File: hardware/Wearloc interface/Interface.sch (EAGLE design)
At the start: 21 parts, among them U1 PCA9306DCT, U2 LTC2804-1GN, U3 TXB0104D

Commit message: interface board work in progress
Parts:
- added C10, C9: (no value), rcl:C-EUC0805K
- added R10, R8, R9: (no value), rcl:R-EU_R0805
- added U4: MCP1826ADJ, wearloc:MCP1826ADJ
- added USB2: MOLEX-47346-0001, wearloc:MOLEX-47346-0001
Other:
- note added: "Jennifer Nist Universität Freiburg"
- note added: "Logic converters"
- note added: "Power supply and connectors"
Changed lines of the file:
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@@
 <part name="R6" library="rcl" deviceset="R-EU_" device="R0805"/>
 <part name="R7" library="rcl" deviceset="R-EU_" device="R0805"/>
+<part name="FRAME1" library="frames" deviceset="A4L-LOC" device=""/>
+<part name="FRAME2" library="frames" deviceset="A4L-LOC" device=""/>
+<part name="USB2" library="wearloc" deviceset="MOLEX-47346-0001" device=""/>
+<part name="U4" library="wearloc" deviceset="MCP1826" device="ADJ"/>
 <part name="JP1" library="wearloc" deviceset="INTEL_EDISON_BB_HEADER" device=""/>
-<part name="FRAME1" library="frames" deviceset="A4L-LOC" device=""/>
 <part name="USB1" library="wearloc" deviceset="MOLEX-47346-0001" device=""/>
+<part name="R8" library="rcl" deviceset="R-EU_" device="R0805"/>
+<part name="R9" library="rcl" deviceset="R-EU_" device="R0805"/>
+<part name="R10" library="rcl" deviceset="R-EU_" device="R0805"/>
+<part name="C9" library="rcl" deviceset="C-EU" device="C0805K"/>
+<part name="C10" library="rcl" deviceset="C-EU" device="C0805K"/>
 </parts>
 <sheets>
 <sheet>
 <plain>
+<text x="165.1" y="10.16" size="3.81" layer="94">Jennifer Nist
+Universität Freiburg</text>
+<text x="217.17" y="20.32" size="2.1844" layer="94">Logic converters</text>
 </plain>
 <instances>
-<instance part="U1" gate="PCA9306" x="50.8" y="160.02"/>
-<instance part="U2" gate="LTC2804-1" x="33.02" y="45.72"/>
-<instance part="U3" gate="TXB0104" x="25.4" y="121.92"/>
-<instance part="C1" gate="G$1" x="68.58" y="139.7"/>
-<instance part="R1" gate="G$1" x="83.82" y="96.52"/>
-<instance part="L1" gate="LQH2MC" x="71.12" y="60.96" rot="R90"/>
-<instance part="C2" gate="G$1" x="68.58" y="129.54"/>
-<instance part="C3" gate="G$1" x="68.58" y="119.38"/>
-<instance part="C4" gate="G$1" x="68.58" y="109.22"/>
-<instance part="C5" gate="G$1" x="55.88" y="109.22"/>
-<instance part="C6" gate="G$1" x="55.88" y="119.38"/>
-<instance part="C7" gate="G$1" x="55.88" y="129.54"/>
-<instance part="C8" gate="G$1" x="55.88" y="139.7"/>
-<instance part="R2" gate="G$1" x="83.82" y="88.9"/>
-<instance part="R3" gate="G$1" x="83.82" y="81.28"/>
-<instance part="R4" gate="G$1" x="83.82" y="73.66"/>
-<instance part="R5" gate="G$1" x="71.12" y="73.66"/>
-<instance part="R6" gate="G$1" x="71.12" y="81.28"/>
-<instance part="R7" gate="G$1" x="71.12" y="88.9"/>
-<instance part="JP1" gate="J17" x="111.76" y="45.72"/>
-<instance part="JP1" gate="J18" x="142.24" y="45.72"/>
-<instance part="JP1" gate="J19" x="177.8" y="45.72"/>
-<instance part="JP1" gate="J20" x="215.9" y="45.72"/>
+<instance part="U1" gate="PCA9306" x="203.2" y="134.62"/>
+<instance part="U2" gate="LTC2804-1" x="33.02" y="114.3"/>
+<instance part="U3" gate="TXB0104" x="142.24" y="68.58"/>
+<instance part="C1" gate="G$1" x="25.4" y="165.1"/>
+<instance part="R1" gate="G$1" x="60.96" y="152.4"/>
+<instance part="L1" gate="LQH2MC" x="38.1" y="152.4" rot="R90"/>
+<instance part="C2" gate="G$1" x="38.1" y="165.1"/>
+<instance part="C3" gate="G$1" x="53.34" y="165.1"/>
+<instance part="C4" gate="G$1" x="68.58" y="165.1"/>
+<instance part="C5" gate="G$1" x="83.82" y="165.1"/>
+<instance part="C6" gate="G$1" x="231.14" y="162.56"/>
+<instance part="C7" gate="G$1" x="170.18" y="83.82"/>
+<instance part="C8" gate="G$1" x="182.88" y="83.82"/>
+<instance part="R2" gate="G$1" x="180.34" y="165.1"/>
+<instance part="R3" gate="G$1" x="180.34" y="157.48"/>
+<instance part="R4" gate="G$1" x="195.58" y="165.1"/>
+<instance part="R5" gate="G$1" x="195.58" y="157.48"/>
+<instance part="R6" gate="G$1" x="213.36" y="165.1"/>
+<instance part="R7" gate="G$1" x="175.26" y="71.12"/>
 <instance part="FRAME1" gate="G$1" x="0" y="0"/>
-<instance part="USB1" gate="MICRO-USB" x="99.06" y="147.32"/>
+</instances>
+<busses>
+</busses>
+<nets>
+</nets>
+</sheet>
+<sheet>
+<plain>
+<text x="165.1" y="10.16" size="3.81" layer="94">Jennifer Nist
+Universität Freiburg</text>
+<text x="215.9" y="20.32" size="2.1844" layer="94">Power supply and connectors</text>
+</plain>
+<instances>
+<instance part="FRAME2" gate="G$1" x="0" y="0"/>
+<instance part="USB2" gate="MICRO-USB" x="-33.02" y="144.78"/>
+<instance part="U4" gate="MCP1826" x="172.72" y="139.7"/>
+<instance part="JP1" gate="J17" x="48.26" y="40.64"/>
+<instance part="JP1" gate="J18" x="78.74" y="40.64"/>
+<instance part="JP1" gate="J19" x="114.3" y="40.64"/>
+<instance part="JP1" gate="J20" x="152.4" y="40.64"/>
+<instance part="USB1" gate="MICRO-USB" x="35.56" y="142.24"/>
+<instance part="R8" gate="G$1" x="203.2" y="152.4"/>
+<instance part="R9" gate="G$1" x="203.2" y="142.24"/>
+<instance part="R10" gate="G$1" x="203.2" y="132.08"/>
+<instance part="C9" gate="G$1" x="137.16" y="149.86"/>
+<instance part="C10" gate="G$1" x="137.16" y="137.16"/>
 </instances>
 <busses>
@@
 </schematic>
 </drawing>
+<compatibility>
+<note version="6.3" minversion="6.2.2" severity="warning">
+Since Version 6.2.2 text objects can contain more than one line,
+which will not be processed correctly with this version.
+</note>
+</compatibility>
 </eagle>

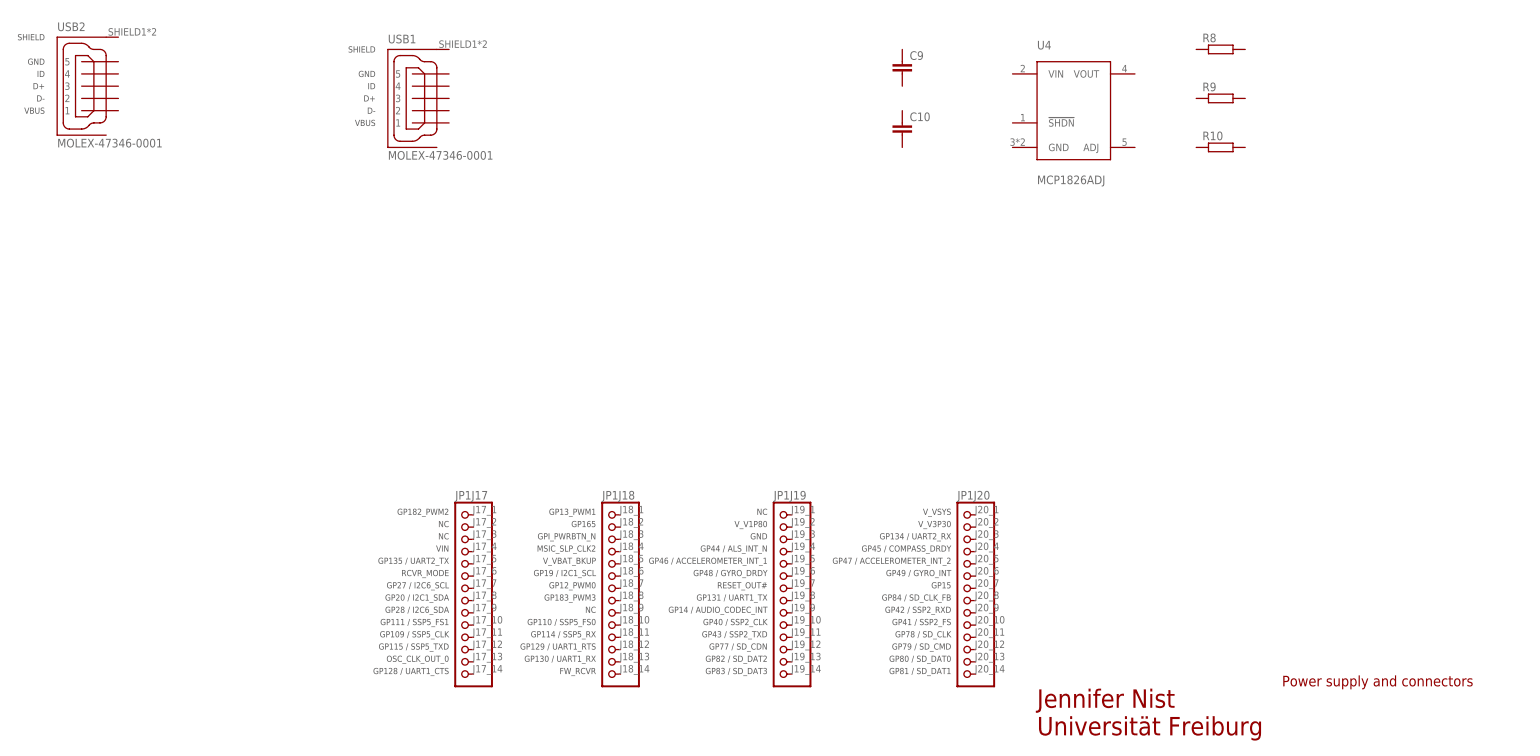
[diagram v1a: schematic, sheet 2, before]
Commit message: worked on schematic
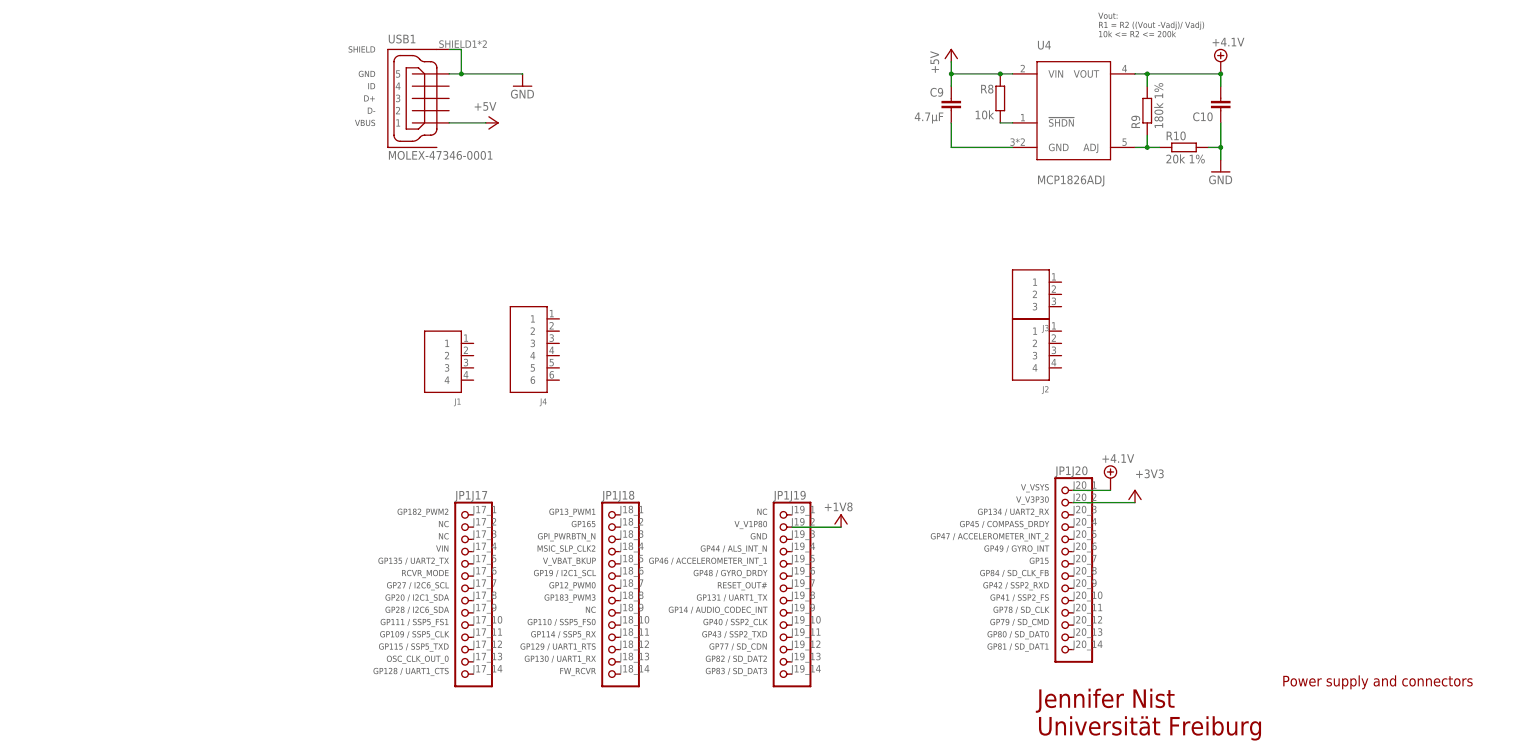
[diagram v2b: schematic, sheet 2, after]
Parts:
- removed USB2: MOLEX-47346-0001, wearloc:MOLEX-47346-0001
- added J1, J2: S4B-XH-A90°, wearloc:S4B-XH-A90°
- added J3: S3B-XH-A90°, wearloc:S3B-XH-A90°
- added J4: S6B-XH-A90°, wearloc:S6B-XH-A90°
- C9: value (none) -> 4.7µF
- R10: value (none) -> 20k 1%
- R8: value (none) -> 10k
- R9: value (none) -> 180k 1%
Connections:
- new net +1V8: JP1J19.2
- new net +3V3: JP1J20.2
- new net +4.1V: C10.2, JP1J20.1, R9.2, U4.VOUT
- new net +5V: C9.1, R8.2, U4.VIN, USB1.1
- new net GND: C10.1, R10.2, USB1.5, USB1.SHIELD
- new net N$1: C9.2, U4.GND
- new net N$2: R8.1, U4.!SHDN
- new net N$4: R10.1, R9.1, U4.ADJ
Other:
- note added: "Vout: R1 = R2 ((Vout -Vadj)/ Vadj) 10k <= R2 <= 200k"
- moved on the sheet: C10, C9, JP1J20, R10, R8, R9
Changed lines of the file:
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@@
 <part name="FRAME1" library="frames" deviceset="A4L-LOC" device=""/>
 <part name="FRAME2" library="frames" deviceset="A4L-LOC" device=""/>
-<part name="USB2" library="wearloc" deviceset="MOLEX-47346-0001" device=""/>
 <part name="U4" library="wearloc" deviceset="MCP1826" device="ADJ"/>
 <part name="JP1" library="wearloc" deviceset="INTEL_EDISON_BB_HEADER" device=""/>
 <part name="USB1" library="wearloc" deviceset="MOLEX-47346-0001" device=""/>
-<part name="R8" library="rcl" deviceset="R-EU_" device="R0805"/>
-<part name="R9" library="rcl" deviceset="R-EU_" device="R0805"/>
-<part name="R10" library="rcl" deviceset="R-EU_" device="R0805"/>
-<part name="C9" library="rcl" deviceset="C-EU" device="C0805K"/>
+<part name="R8" library="rcl" deviceset="R-EU_" device="R0805" value="10k"/>
+<part name="R9" library="rcl" deviceset="R-EU_" device="R0805" value="180k 1%"/>
+<part name="R10" library="rcl" deviceset="R-EU_" device="R0805" value="20k 1%"/>
+<part name="C9" library="rcl" deviceset="C-EU" device="C0805K" value="4.7µF"/>
 <part name="C10" library="rcl" deviceset="C-EU" device="C0805K"/>
+<part name="J1" library="wearloc" deviceset="S4B-XH-A" device="90°"/>
+<part name="J2" library="wearloc" deviceset="S4B-XH-A" device="90°"/>
+<part name="J3" library="wearloc" deviceset="S3B-XH-A" device="90°"/>
+<part name="J4" library="wearloc" deviceset="S6B-XH-A" device="90°"/>
+<part name="P+1" library="supply1" deviceset="+5V" device=""/>
+<part name="GND1" library="supply1" deviceset="GND" device=""/>
+<part name="P+2" library="supply1" deviceset="+5V" device=""/>
+<part name="GND2" library="supply1" deviceset="GND" device=""/>
+<part name="SUPPLY1" library="supply2" deviceset="+4.1V" device=""/>
+<part name="SUPPLY2" library="supply2" deviceset="+4.1V" device=""/>
+<part name="+3V1" library="supply1" deviceset="+3V3" device=""/>
+<part name="+1V1" library="wearloc" deviceset="+1V8" device=""/>
 </parts>
 <sheets>
@@
 Universität Freiburg</text>
 <text x="215.9" y="20.32" size="2.1844" layer="94">Power supply and connectors</text>
+<text x="177.8" y="154.94" size="1.27" layer="97">Vout:
+R1 = R2 ((Vout -Vadj)/ Vadj)
+10k &lt;= R2 &lt;= 200k</text>
 </plain>
 <instances>
 <instance part="FRAME2" gate="G$1" x="0" y="0"/>
-<instance part="USB2" gate="MICRO-USB" x="-33.02" y="144.78"/>
 <instance part="U4" gate="MCP1826" x="172.72" y="139.7"/>
 <instance part="JP1" gate="J17" x="48.26" y="40.64"/>
 <instance part="JP1" gate="J18" x="78.74" y="40.64"/>
 <instance part="JP1" gate="J19" x="114.3" y="40.64"/>
-<instance part="JP1" gate="J20" x="152.4" y="40.64"/>
+<instance part="JP1" gate="J20" x="172.72" y="45.72"/>
 <instance part="USB1" gate="MICRO-USB" x="35.56" y="142.24"/>
-<instance part="R8" gate="G$1" x="203.2" y="152.4"/>
-<instance part="R9" gate="G$1" x="203.2" y="142.24"/>
-<instance part="R10" gate="G$1" x="203.2" y="132.08"/>
-<instance part="C9" gate="G$1" x="137.16" y="149.86"/>
-<instance part="C10" gate="G$1" x="137.16" y="137.16"/>
+<instance part="R8" gate="G$1" x="157.48" y="142.24" smashed="yes" rot="R90">
+<attribute name="NAME" x="156.21" y="143.2814" size="1.778" layer="95" rot="MR0"/>
+<attribute name="VALUE" x="156.21" y="137.922" size="1.778" layer="96" rot="MR0"/>
+</instance>
+<instance part="R9" gate="G$1" x="187.96" y="139.7" rot="R90"/>
+<instance part="R10" gate="G$1" x="195.58" y="132.08"/>
+<instance part="C9" gate="G$1" x="147.32" y="142.24" smashed="yes">
+<attribute name="NAME" x="145.796" y="142.621" size="1.778" layer="95" rot="MR0"/>
+<attribute name="VALUE" x="145.796" y="137.541" size="1.778" layer="96" rot="MR0"/>
+</instance>
+<instance part="C10" gate="G$1" x="203.2" y="139.7" rot="R180"/>
+<instance part="J1" gate="JST_XH" x="43.18" y="88.9"/>
+<instance part="J2" gate="JST_XH" x="165.1" y="91.44"/>
+<instance part="J3" gate="JST_XH" x="165.1" y="101.6"/>
+<instance part="J4" gate="JST_XH" x="60.96" y="91.44"/>
+<instance part="P+1" gate="1" x="53.34" y="137.16" rot="R270"/>
+<instance part="GND1" gate="1" x="58.42" y="144.78"/>
+<instance part="P+2" gate="1" x="147.32" y="152.4"/>
+<instance part="GND2" gate="1" x="203.2" y="127"/>
+<instance part="SUPPLY1" gate="P" x="203.2" y="149.86"/>
+<instance part="SUPPLY2" gate="P" x="180.34" y="63.5"/>
+<instance part="+3V1" gate="G$1" x="185.42" y="60.96" smashed="yes">
+<attribute name="VALUE" x="185.42" y="63.5" size="1.778" layer="96"/>
+</instance>
+<instance part="+1V1" gate="G$1" x="124.46" y="55.88" smashed="yes">
+<attribute name="VALUE" x="127" y="58.42" size="1.778" layer="96" rot="R180"/>
+</instance>
 </instances>
 <busses>
 </busses>
 <nets>
+<net name="+5V" class="0">
+<segment>
+<pinref part="USB1" gate="MICRO-USB" pin="1"/>
+<pinref part="P+1" gate="1" pin="+5V"/>
+<wire x1="43.18" y1="137.16" x2="50.8" y2="137.16" width="0.1524" layer="91"/>
+</segment>
+<segment>
+<pinref part="U4" gate="MCP1826" pin="VIN"/>
+<pinref part="P+2" gate="1" pin="+5V"/>
+<wire x1="160.02" y1="147.32" x2="157.48" y2="147.32" width="0.1524" layer="91"/>
+<pinref part="C9" gate="G$1" pin="1"/>
+<wire x1="157.48" y1="147.32" x2="147.32" y2="147.32" width="0.1524" layer="91"/>
+<wire x1="147.32" y1="147.32" x2="147.32" y2="149.86" width="0.1524" layer="91"/>
+<wire x1="147.32" y1="144.78" x2="147.32" y2="147.32" width="0.1524" layer="91"/>
+<junction x="147.32" y="147.32"/>
+<pinref part="R8" gate="G$1" pin="2"/>
+<junction x="157.48" y="147.32"/>
+</segment>
+</net>
+<net name="GND" class="0">
+<segment>
+<pinref part="USB1" gate="MICRO-USB" pin="5"/>
+<pinref part="GND1" gate="1" pin="GND"/>
+<wire x1="43.18" y1="147.32" x2="45.72" y2="147.32" width="0.1524" layer="91"/>
+<pinref part="USB1" gate="MICRO-USB" pin="SHIELD"/>
+<wire x1="45.72" y1="147.32" x2="58.42" y2="147.32" width="0.1524" layer="91"/>
+<wire x1="43.18" y1="152.4" x2="45.72" y2="152.4" width="0.1524" layer="91"/>
+<wire x1="45.72" y1="152.4" x2="45.72" y2="147.32" width="0.1524" layer="91"/>
+<junction x="45.72" y="147.32"/>
+</segment>
+<segment>
+<pinref part="R10" gate="G$1" pin="2"/>
+<wire x1="200.66" y1="132.08" x2="203.2" y2="132.08" width="0.1524" layer="91"/>
+<pinref part="GND2" gate="1" pin="GND"/>
+<wire x1="203.2" y1="132.08" x2="203.2" y2="129.54" width="0.1524" layer="91"/>
+<pinref part="C10" gate="G$1" pin="1"/>
+<wire x1="203.2" y1="137.16" x2="203.2" y2="132.08" width="0.1524" layer="91"/>
+<junction x="203.2" y="132.08"/>
+</segment>
+</net>
+<net name="N$1" class="0">
+<segment>
+<pinref part="C9" gate="G$1" pin="2"/>
+<wire x1="147.32" y1="137.16" x2="147.32" y2="132.08" width="0.1524" layer="91"/>
+<pinref part="U4" gate="MCP1826" pin="GND"/>
+<wire x1="147.32" y1="132.08" x2="160.02" y2="132.08" width="0.1524" layer="91"/>
+</segment>
+</net>
+<net name="N$2" class="0">
+<segment>
+<pinref part="U4" gate="MCP1826" pin="!SHDN"/>
+<pinref part="R8" gate="G$1" pin="1"/>
+<wire x1="160.02" y1="137.16" x2="157.48" y2="137.16" width="0.1524" layer="91"/>
+</segment>
+</net>
+<net name="N$4" class="0">
+<segment>
+<pinref part="R9" gate="G$1" pin="1"/>
+<wire x1="187.96" y1="134.62" x2="187.96" y2="132.08" width="0.1524" layer="91"/>
+<pinref part="U4" gate="MCP1826" pin="ADJ"/>
+<wire x1="187.96" y1="132.08" x2="185.42" y2="132.08" width="0.1524" layer="91"/>
+<pinref part="R10" gate="G$1" pin="1"/>
+<wire x1="187.96" y1="132.08" x2="190.5" y2="132.08" width="0.1524" layer="91"/>
+<junction x="187.96" y="132.08"/>
+</segment>
+</net>
+<net name="+4.1V" class="0">
+<segment>
+<pinref part="R9" gate="G$1" pin="2"/>
+<wire x1="187.96" y1="144.78" x2="187.96" y2="147.32" width="0.1524" layer="91"/>
+<pinref part="U4" gate="MCP1826" pin="VOUT"/>
+<wire x1="187.96" y1="147.32" x2="185.42" y2="147.32" width="0.1524" layer="91"/>
+<wire x1="187.96" y1="147.32" x2="203.2" y2="147.32" width="0.1524" layer="91"/>
+<junction x="187.96" y="147.32"/>
+<pinref part="C10" gate="G$1" pin="2"/>
+<wire x1="203.2" y1="147.32" x2="203.2" y2="144.78" width="0.1524" layer="91"/>
+<pinref part="SUPPLY1" gate="P" pin="+4.1V"/>
+<junction x="203.2" y="147.32"/>
+</segment>
+<segment>
+<pinref part="JP1" gate="J20" pin="1"/>
+<pinref part="SUPPLY2" gate="P" pin="+4.1V"/>
+<wire x1="172.72" y1="60.96" x2="180.34" y2="60.96" width="0.1524" layer="91"/>
+</segment>
+</net>
+<net name="+3V3" class="0">
+<segment>
+<pinref part="JP1" gate="J20" pin="2"/>
+<wire x1="172.72" y1="58.42" x2="185.42" y2="58.42" width="0.1524" layer="91"/>
+<pinref part="+3V1" gate="G$1" pin="+3V3"/>
+</segment>
+</net>
+<net name="+1V8" class="0">
+<segment>
+<pinref part="JP1" gate="J19" pin="2"/>
+<wire x1="114.3" y1="53.34" x2="124.46" y2="53.34" width="0.1524" layer="91"/>
+<pinref part="+1V1" gate="G$1" pin="+1V8"/>
+</segment>
+</net>
 </nets>
 </sheet>
